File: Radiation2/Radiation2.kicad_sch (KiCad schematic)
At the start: 0 parts

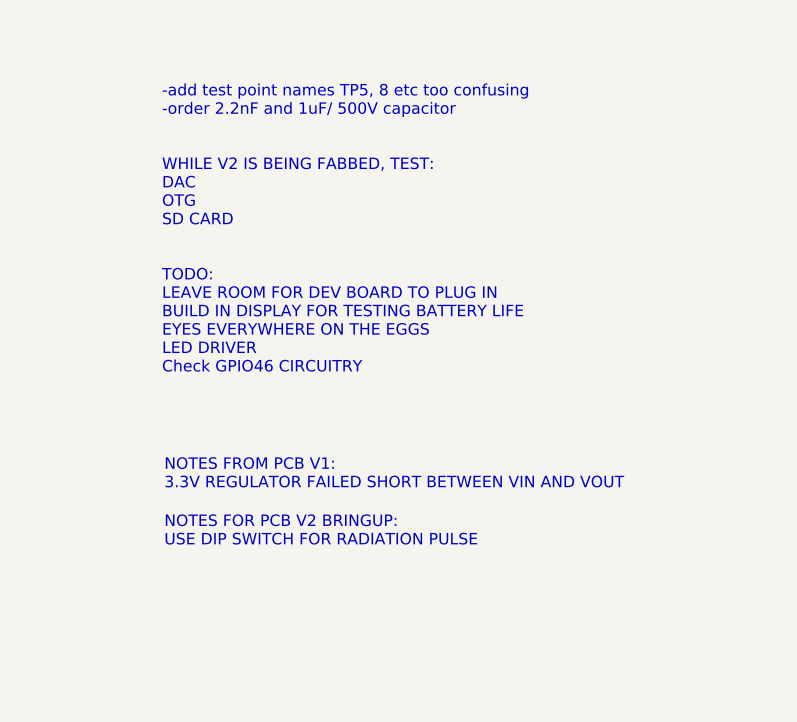
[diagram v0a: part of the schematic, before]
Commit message: Adding V3
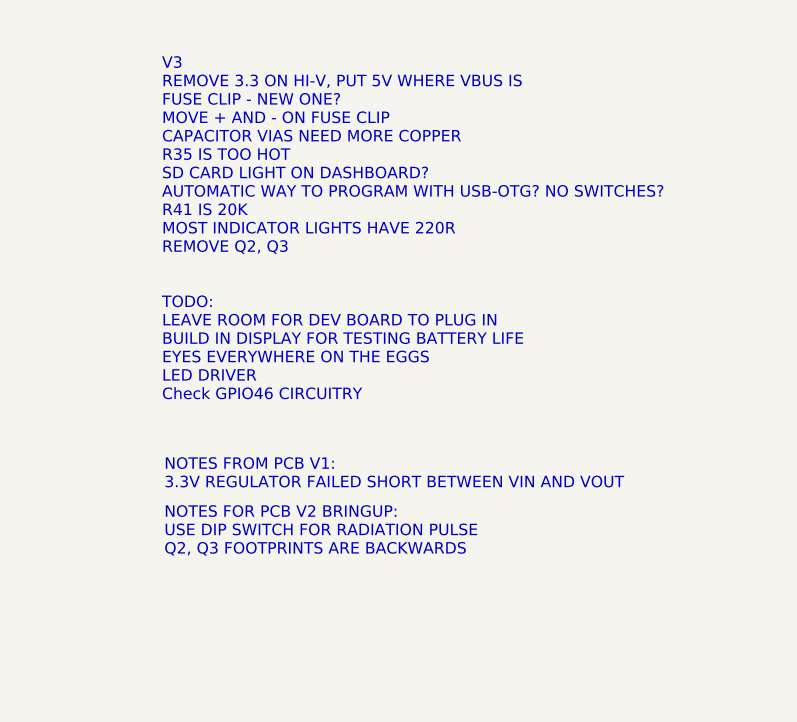
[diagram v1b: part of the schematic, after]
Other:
- note added: "NOTES FOR PCB V2 BRINGUP: USE DIP SWITCH FOR RADIATION PULSE Q2, Q3 FOOTPRINTS ARE BACKWARDS"
- note added: "V3 REMOVE 3.3 ON HI-V, PUT 5V WHERE VBUS IS FUSE CLIP - NEW ONE? MOVE + AND - ON FUSE CLIP CAPACITOR VIAS NEED MORE COPPER R35 IS TOO HOT SD CARD LIGHT ON DASHBOARD? AUTOMATIC WAY TO PROGRAM WITH USB-OTG? NO SWITCHES? R41 IS 20K MOST INDICATOR LIGHTS HAVE 220R REMOVE Q2, Q3 TODO: LEAVE ROOM FOR DEV BOARD TO PLUG IN BUILD IN DISPLAY FOR TESTING BATTERY LIFE EYES EVERYWHERE ON THE EGGS LED DRIVER C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"
- note removed: "-add test point names TP5, 8 etc too confusing -order 2.2nF and 1uF/ 500V capacitor WHILE V2 IS BEING FABBED, TEST: DAC OTG SD CARD TODO: LEAVE ROOM FOR DEV BOARD TO PLUG IN BUILD IN DISPLAY FOR TESTING BATTERY LIFE EYES EVERYWHERE ON THE EGGS LED DRIVER Check GPIO46 CIRCUITRY"
- note removed: "NOTES FOR PCB V2 BRINGUP: USE DIP SWITCH FOR RADIATION PULSE"
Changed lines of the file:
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@@
 		(title "POWER")
 	)
-	(text "-add test point names TP5, 8 etc too confusing\n-order 2.2nF and 1uF/ 500V capacitor\n\n\nWHILE V2 IS BEING FABBED, TEST:\nDAC\nOTG\nSD CARD\n\n\nTODO:\nLEAVE ROOM FOR DEV BOARD TO PLUG IN\nBUILD IN DISPLAY FOR TESTING BATTERY LIFE\nEYES EVERYWHERE ON THE EGGS\nLED DRIVER\nCheck GPIO46 CIRCUITRY"
+	(text "V3\nREMOVE 3.3 ON HI-V, PUT 5V WHERE VBUS IS\nFUSE CLIP - NEW ONE?\nMOVE + AND - ON FUSE CLIP\nCAPACITOR VIAS NEED MORE COPPER\nR35 IS TOO HOT\nSD CARD LIGHT ON DASHBOARD?\nAUTOMATIC WAY TO PROGRAM WITH USB-OTG? NO SWITCHES?\nR41 IS 20K\nMOST INDICATOR LIGHTS HAVE 220R \nREMOVE Q2, Q3\n\n\nTODO:\nLEAVE ROOM FOR DEV BOARD TO PLUG IN\nBUILD IN DISPLAY FOR TESTING BATTERY LIFE\nEYES EVERYWHERE ON THE EGGS\nLED DRIVER\nCheck GPIO46 CIRCUITRY"
 		(exclude_from_sim no)
 		(at 186.436 53.848 0)
@@
 		)
 	)
-	(text "NOTES FOR PCB V2 BRINGUP:\nUSE DIP SWITCH FOR RADIATION PULSE"
+	(text "NOTES FOR PCB V2 BRINGUP:\nUSE DIP SWITCH FOR RADIATION PULSE\nQ2, Q3 FOOTPRINTS ARE BACKWARDS\n"
 		(exclude_from_sim no)
 		(at 186.69 87.376 0)
